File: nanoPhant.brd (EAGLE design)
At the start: 36.2 x 34.9 mm, 45 parts, among them J1 AMP FCI 10103594-0001LF, U3 ATMEGA32U4, Y1 16MHz

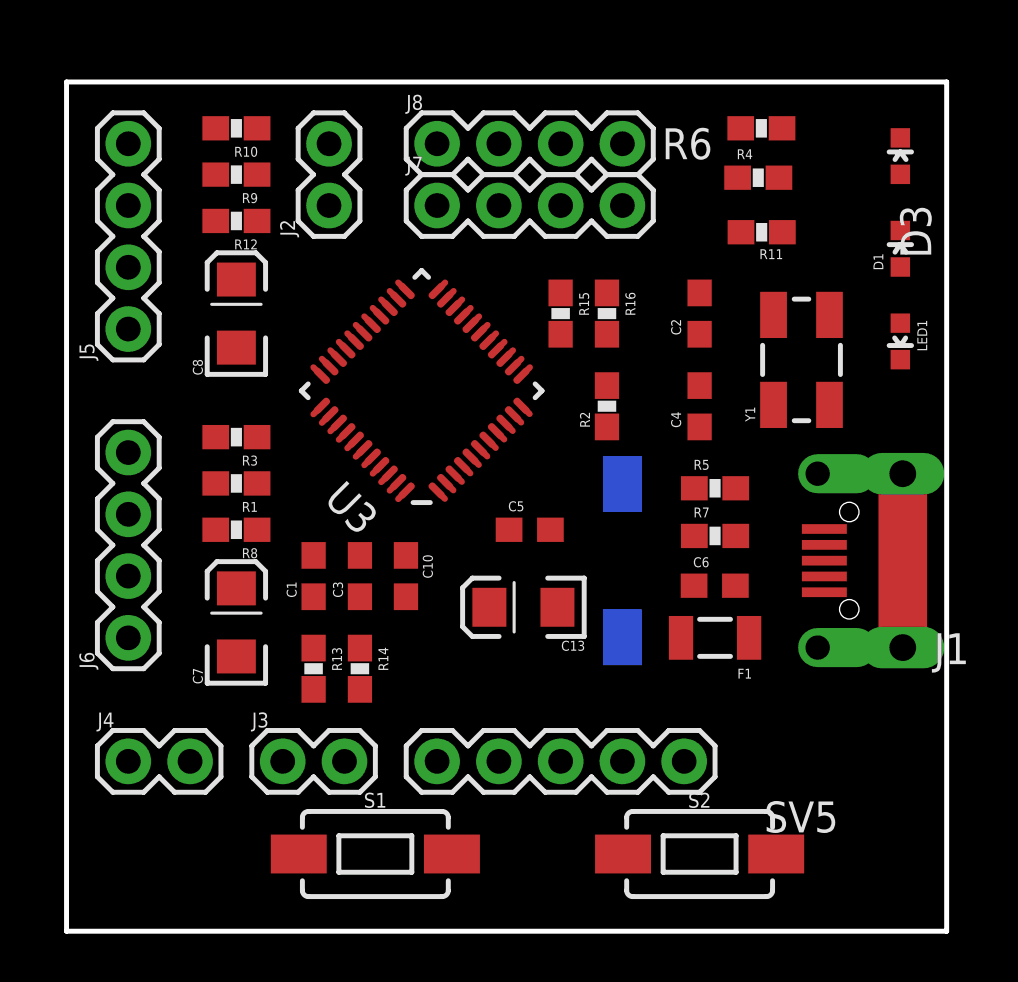
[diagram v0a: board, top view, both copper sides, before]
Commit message: Routed and Gerber files
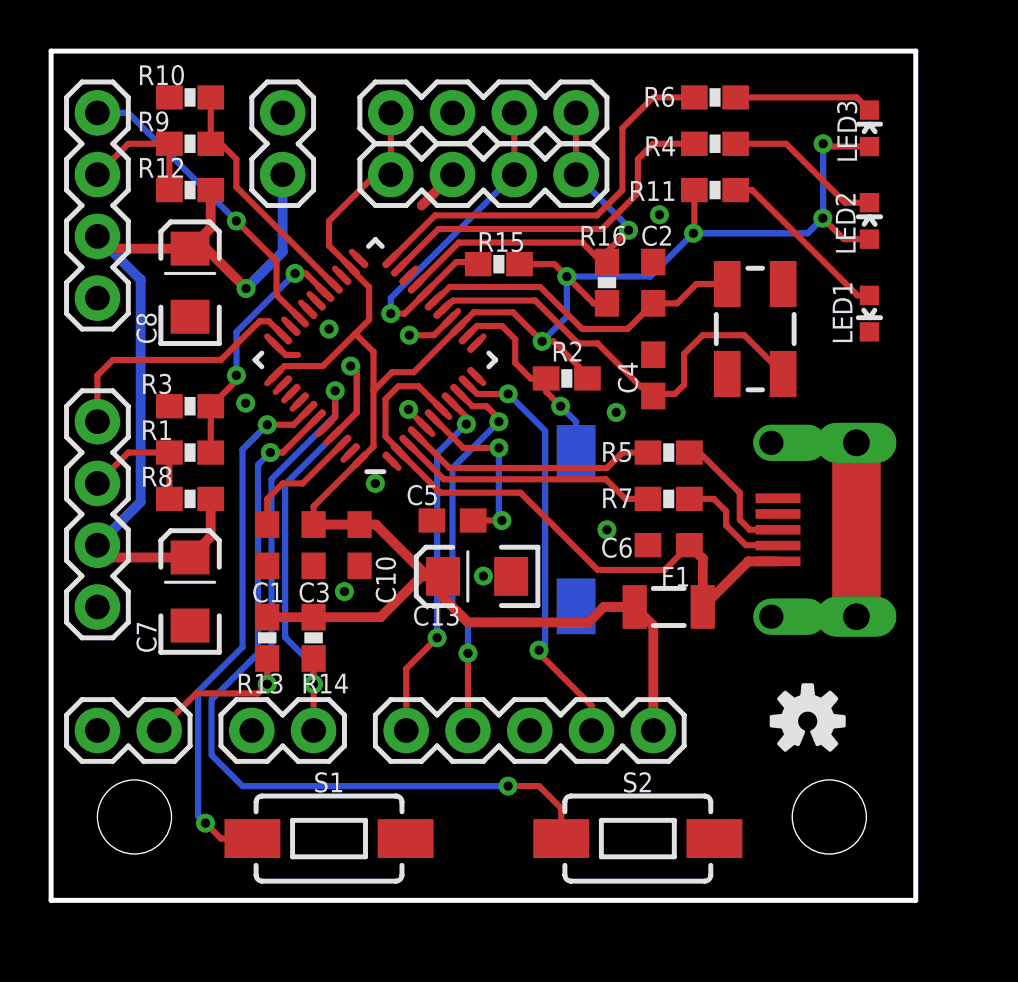
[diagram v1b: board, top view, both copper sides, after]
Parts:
- removed D1: Yellow, SparkFun:LED-0603
- removed D3: Green, SparkFun:LED-0603
- added LED2: Yellow, SparkFun:LED-0603
- added LED3: Red, SparkFun:LED-0603
- added U$1: OSHW-LOGOS, SparkFun:OSHW-LOGO-S
- LED1: value Red -> Blue
- R11: value 1K -> 330
- moved U$3 28.5 mm to (31.1, 7.37)
- moved J2 4.26 mm to (9.53, 32.4), turned to 270 degrees
- moved R15 3.25 mm to (18.4, 26.2), turned to 0 degrees
- moved C5 3.20 mm to (16.5, 15.6)
- moved S2 2.62 mm to (24.1, 2.54)
- moved R11 2.59 mm to (27.3, 29.2)
- moved C6 2.52 mm to (25.4, 14.6)
- moved R7 2.44 mm to (25.4, 16.5)
- moved R5 2.41 mm to (25.4, 18.4)
- moved R6 2.29 mm to (27.3, 33.0)
- moved R10 2.29 mm to (5.71, 33.0)
- moved C2 2.29 mm to (24.8, 25.4)
- moved C4 2.29 mm to (24.8, 21.6)
- moved F1 2.29 mm to (25.4, 12.1)
- moved R8 2.29 mm to (5.71, 16.5)
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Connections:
- removed net N$11: J7.2
- net GND: now also J1.P$1, J1.P$2, J1.P$3, J1.P$4, J1.P$5, J7.2
- net N$5: now also LED2.C; no longer D1.C
- net N$7: now also LED3.C; no longer D3.C
- net VCC: now also LED2.A, LED3.A; no longer D1.A, D3.A
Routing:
- net VCC: track 0.00 -> 92.8 mm, vias 0 -> 5
- net +12V: track 0.00 -> 36.0 mm, vias 0 -> 1
- net SW2: track 0.00 -> 32.5 mm, vias 0 -> 2
- net UVCC: track 0.00 -> 26.3 mm
- net SW1: track 0.00 -> 21.9 mm, vias 0 -> 2
- net TEMP1: track 0.00 -> 21.1 mm, vias 0 -> 2
- net TEMP2: track 0.00 -> 21.1 mm, vias 0 -> 2
- net N$1: track 0.00 -> 18.3 mm
- net MOSI: track 0.00 -> 17.4 mm, vias 0 -> 2
- net TXLED: track 0.00 -> 16.8 mm
- net I2C_SDA: track 0.00 -> 16.3 mm, vias 0 -> 1
- net SCK: track 0.00 -> 16.0 mm, vias 0 -> 2
- net N$3: track 0.00 -> 15.1 mm
- net MISO: track 0.00 -> 14.9 mm, vias 0 -> 2
- net I2C_SCL: track 0.00 -> 14.9 mm, vias 0 -> 1
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- added copper zone on layer 1, net GND
- added copper zone on layer 16, net GND
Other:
- board size 36.2 x 34.9 mm -> 35.6 x 34.9 mm
- board text added: "1"
- board text added: "12V"
- board text added: "5V"
- board text added: "FAN1"
- board text added: "FAN2"
- board text added: "GND"
- board text added: "MISO"
- board text added: "MOSI"
- board text added: "RESET"
- board text added: "SCK"
- board text added: "SCL"
- board text added: "SDA"
- board text added: "T1"
- board text added: "T2"
- board text added: "nanoPhant"
- board text added: "psyte / Patrik Marcacci - 2018"
- board text removed: "3.3V Reg / 8MHz"
- board text removed: "5V Reg / 16MHz"
- board text removed: "Mark back accordingly"
- board text removed: "Valid combinations:"
